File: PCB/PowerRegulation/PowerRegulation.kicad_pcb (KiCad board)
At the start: 4 copper layers, 128 x 66.5 mm, 138 parts, among them J1 USB_C_Receptacle_USB2.0_14P, J3 Wii audio in, J4 OLED, SW1 RESET, SW2 BOOT, U1 BQ25883RGER, U10 MCP4651-503E/ST, U11 PAM8403, U2 TPS22918DBVR, U3 STM32F072CBTx, U4 TPS22918DBVR, U5 TPS563200DDCR, U6 TPS563200DDCR, U7 TPS563200DDCR, U8 TPS563200DDCR, U9 TPS563200DDCR

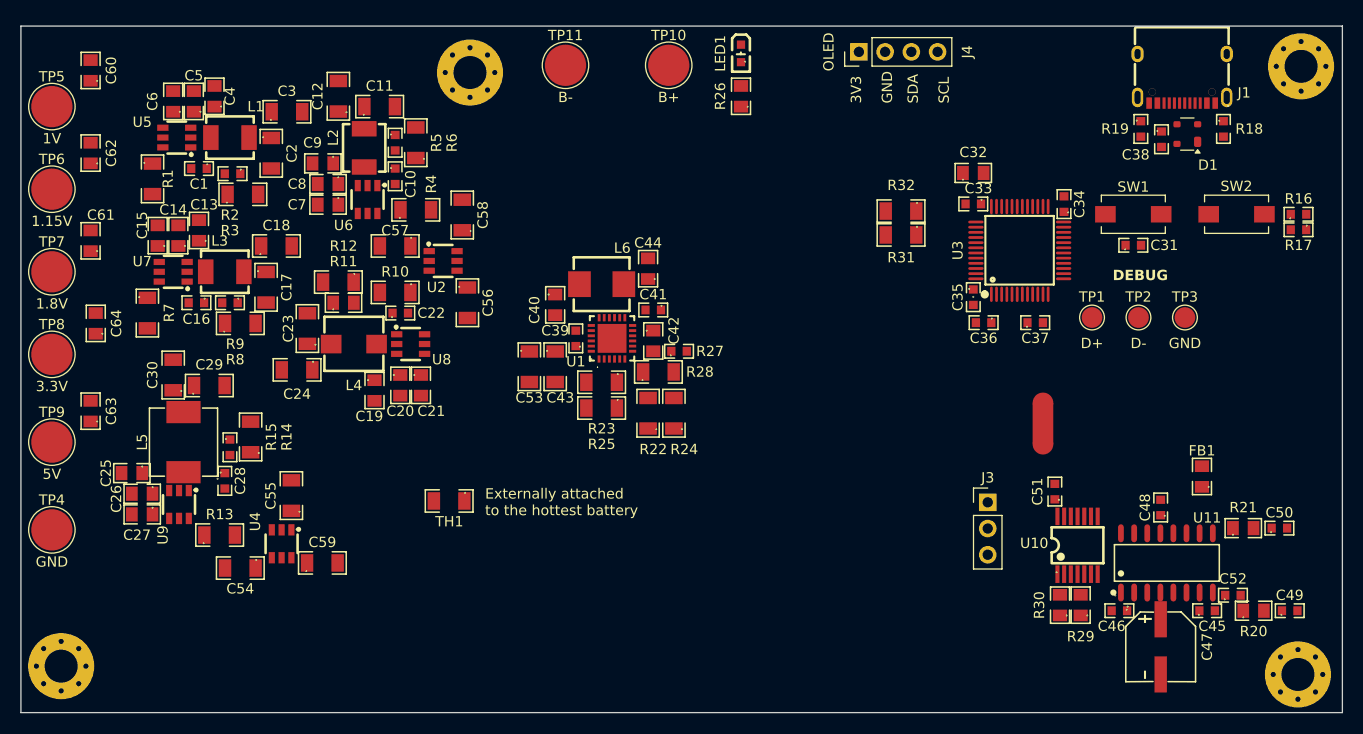
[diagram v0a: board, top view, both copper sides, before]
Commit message: make logo, route some stuff
THIS IS BEFORE THE BATT+ ON In2.Cu
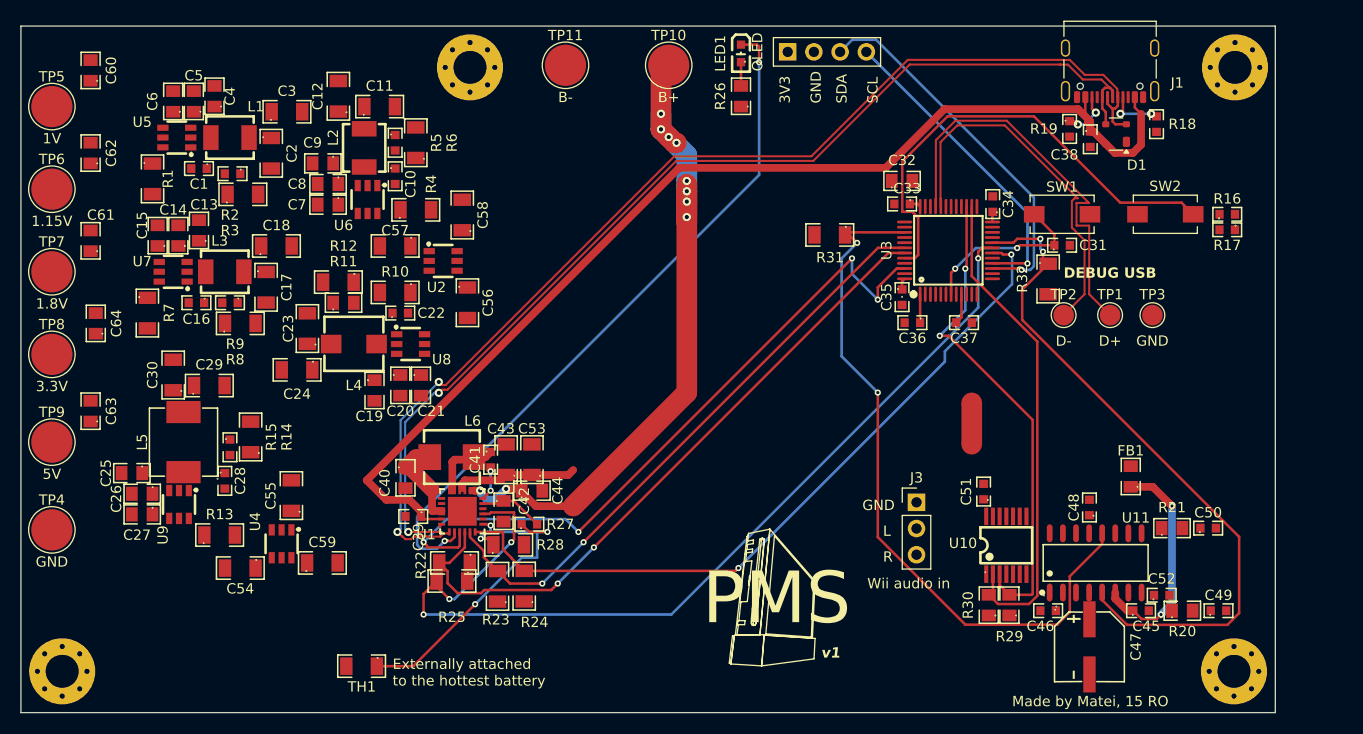
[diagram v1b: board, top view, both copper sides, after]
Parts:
- J1: value USB_C_Receptacle_USB2.0_14P -> USB_C_Receptacle_USB2.0_16P; footprint EasyEDA:USB-C-SMD_TYPE-C-16PIN-2MD-073 -> Connector_USB:USB_C_Receptacle_Palconn_UTC16-G
- moved C44 24.3 mm to (112.0, 113.5), turned to 0 degrees
- moved R22 23.7 mm to (104.5, 120.5), turned to 180 degrees
- moved C39 23.4 mm to (100.5, 116.0), turned to 180 degrees
- moved R23 22.2 mm to (108.7, 122.8), turned to 90 degrees
- moved C40 22.2 mm to (99.8, 112.2)
- moved L6 22.2 mm to (104.2, 110.2)
- moved R24 22.2 mm to (111.2, 122.8)
- moved R25 22.2 mm to (104.2, 122.2)
- moved R27 22.2 mm to (111.8, 116.8)
- moved R28 22.2 mm to (109.8, 118.8)
- moved U1 22.2 mm to (105.2, 115.5)
- moved C42 22.0 mm to (109.2, 115.5)
- moved C41 21.4 mm to (108.0, 110.5), turned to -90 degrees
- moved TH1 18.1 mm to (95.5, 130.5)
- moved R32 15.7 mm to (162.0, 93.0), turned to -90 degrees
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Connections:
- net Net-(U3-PA11) renamed /Debug-
- net Net-(U3-PA12) renamed /Debug+
- J1 pad A8: (no net) -> unconnected-(J1-SBU1-PadA8)
- J1 pad B8: (no net) -> unconnected-(J1-SBU2-PadB8)
- U3 pad 46: unconnected-(U3-PB9-Pad46) -> CE
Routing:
- net VBUS: track 0.00 -> 112.1 mm
- net D-: track 0.00 -> 108.2 mm, vias 0 -> 2
- net D+: track 0.00 -> 104.4 mm, vias 0 -> 2
- net PG_BATT: track 0.00 -> 93.4 mm, vias 0 -> 4
- net INT_BATT: track 0.00 -> 71.4 mm, vias 0 -> 2
- net BATTERY+: track 0.00 -> 69.8 mm, vias 0 -> 10
- net SHDN: track 0.00 -> 69.5 mm, vias 0 -> 2
- net CE: track 0.00 -> 68.7 mm, vias 0 -> 4
- net Net-(LED1-C): track 0.00 -> 68.6 mm, vias 0 -> 2
- net MUTE: track 0.00 -> 66.6 mm, vias 0 -> 2
- net SDA_BATT: track 0.00 -> 65.2 mm, vias 0 -> 2
- net SCL_BATT: track 0.00 -> 58.3 mm, vias 0 -> 2
- net SCL_AUD: track 0.00 -> 47.9 mm
- net SDA_AUD: track 0.00 -> 47.5 mm, vias 0 -> 2
- net BOOT0: track 0.00 -> 45.6 mm
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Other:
- board size 128 x 66.5 mm -> 121.5 x 66.5 mm
- board text added: "DEBUG USB"
- board text added: "L"
- board text added: "Made by Matei, 15 RO"
- board text added: "PMS"
- board text added: "R"
- board text added: "v1"
- board text removed: "DEBUG"
